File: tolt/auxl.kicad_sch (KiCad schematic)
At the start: 2 parts, among them U17 BMI160, U18 ESP32-C3_SUPERMINI_SMD

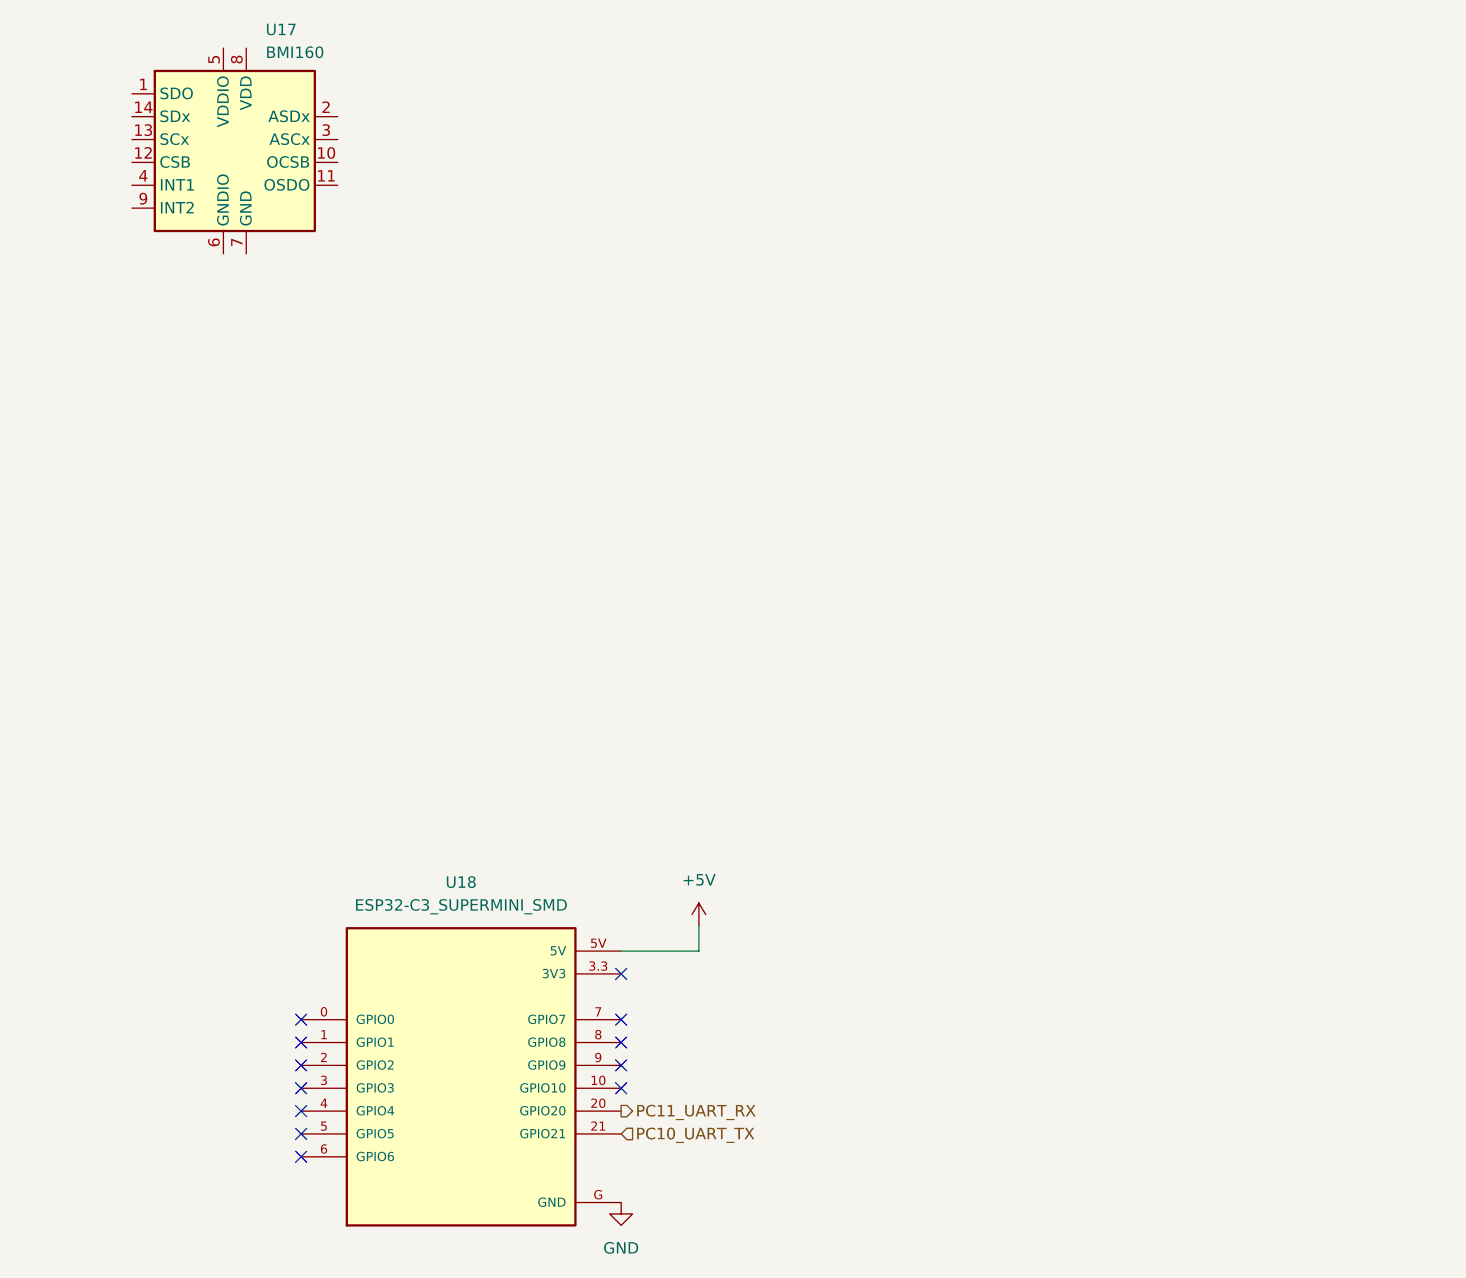
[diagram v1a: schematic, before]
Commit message: Reapply "Merge branch 'main' of https://github.com/LJBoxx/bigtolt"
This reverts commit 10d1035653869a11abcc4dc45a35a471baa73785.
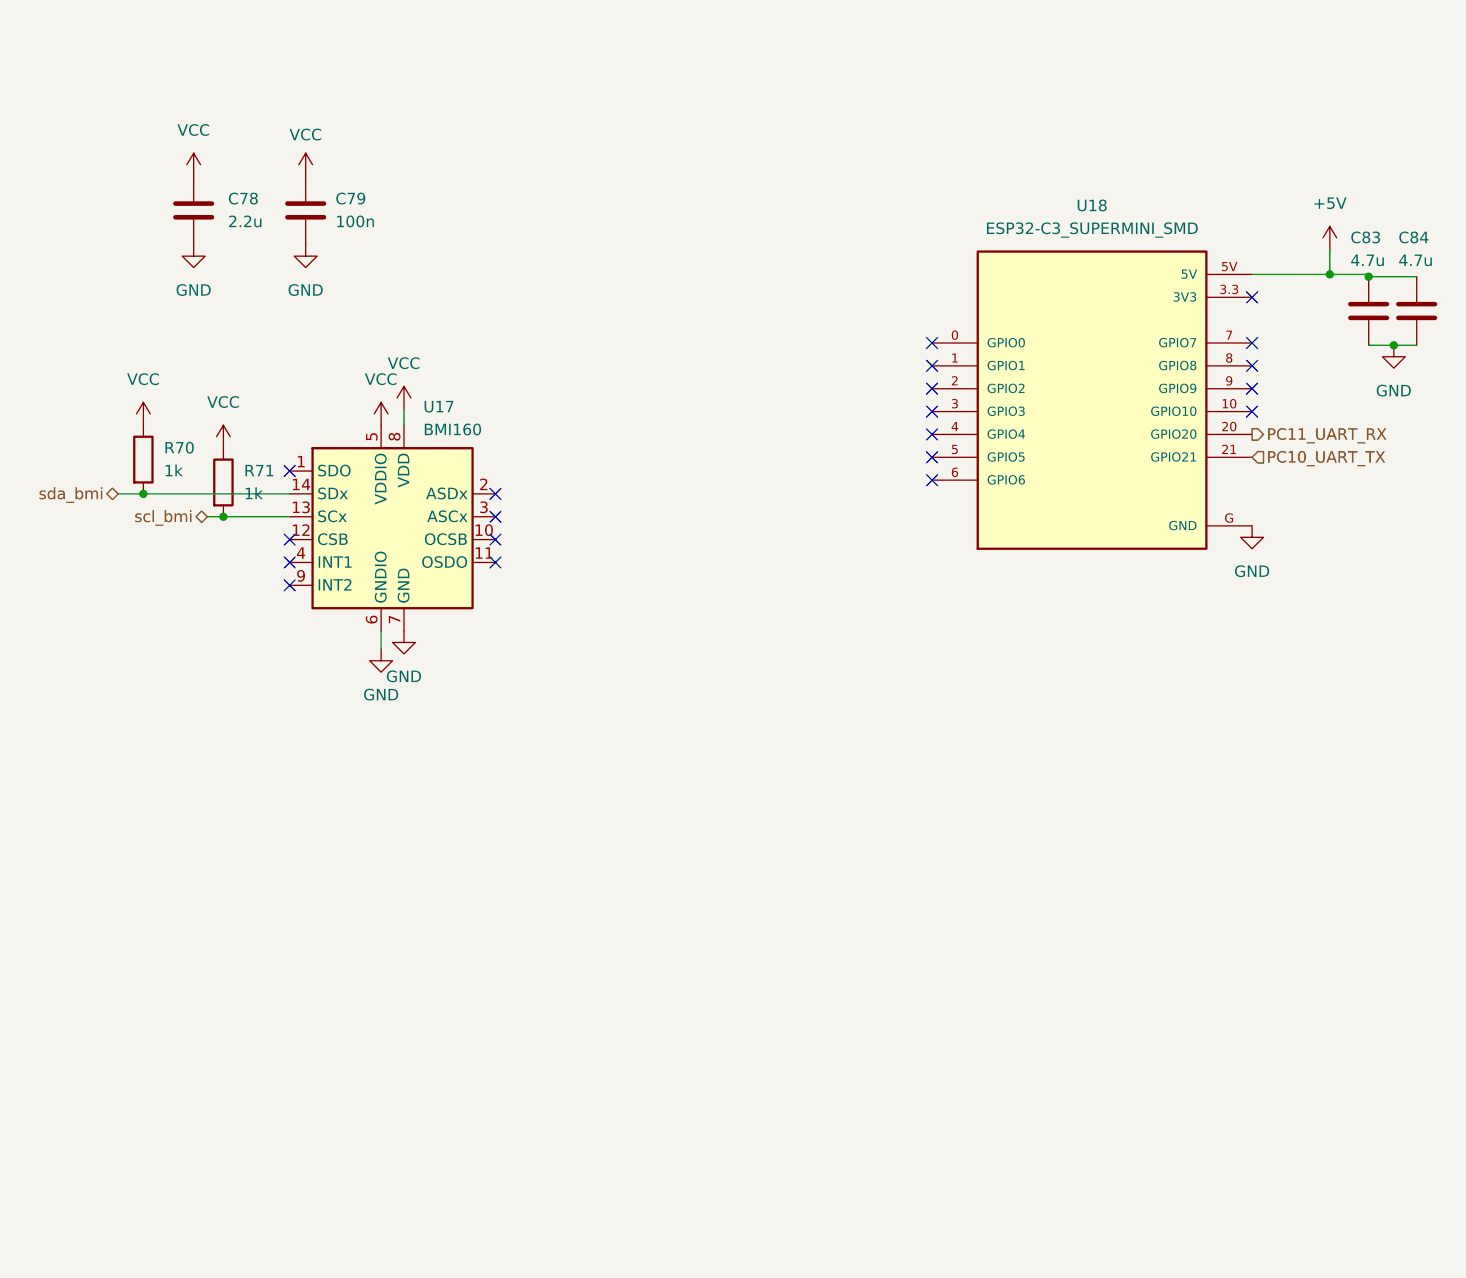
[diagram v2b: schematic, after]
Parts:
- added C78: 2.2u, Capacitor_SMD:C_0603_1608Metric, symbol Device:C
- added C79: 100n, Capacitor_SMD:C_0402_1005Metric, symbol Device:C
- added C83, C84: 4.7u, Capacitor_SMD:C_0805_2012Metric, symbol Device:C
- added R70, R71: 1k, Resistor_SMD:R_0603_1608Metric, symbol Device:R
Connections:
- net +5V: now also C83.2, C84.2
- net GND: now also U17.6 (GNDIO), U17.7 (GND), C78.1, C79.1, C83.1, C84.1
- net scl_bmi: now reaches U17.13 (SCx)
- net scl_bmi: now also R71.2
- net sda_bmi: now reaches U17.14 (SDx)
- net sda_bmi: now also R70.2
- net VCC: now reaches U17.5 (VDDIO)
- net VCC: now also U17.8 (VDD), C78.2, C79.2, R70.1, R71.1
- no-connect marks 12 -> 20
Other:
- moved on the sheet: U17, U18
